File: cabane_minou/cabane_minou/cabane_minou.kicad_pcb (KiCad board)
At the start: 2 copper layers, 140 x 120.1 mm, 137 parts, among them J1 Alim 12V, J10 Serial, J11 LEDs Res, J12 Leds, J13 Buttons, J14 Couvercle, J15 Commande 12V, J2 Log, J3 Screen, J4 Bas, J5 LEDs Bas, J6 Move Tour, J7 LEDs Tour, J8 Move Haut, J9 LEDs Haut, Q1 BPC_2N2222A, Q10 BC327, Q11 BPC_2N2222A, Q12 BPC_2N2222A, Q13 BC327, Q14 BC327, Q2 BC327, Q3 BPC_2N2222A, Q4 BC327, Q5 BPC_2N2222A, Q6 BPC_IPP034N03L, Q7 BPC_2N2222A, Q8 BPC_2N2222A, Q9 BC327, U1 BPC_Alim5V, U2 LM1117DT-3.3, U3 BPC_ATMEGA2560_PRO, U5 RtcArduino, U6 BPC_ESP8266-01_ESP-01, X1 Trou, X2 Trou, X3 Trou, X4 Trou

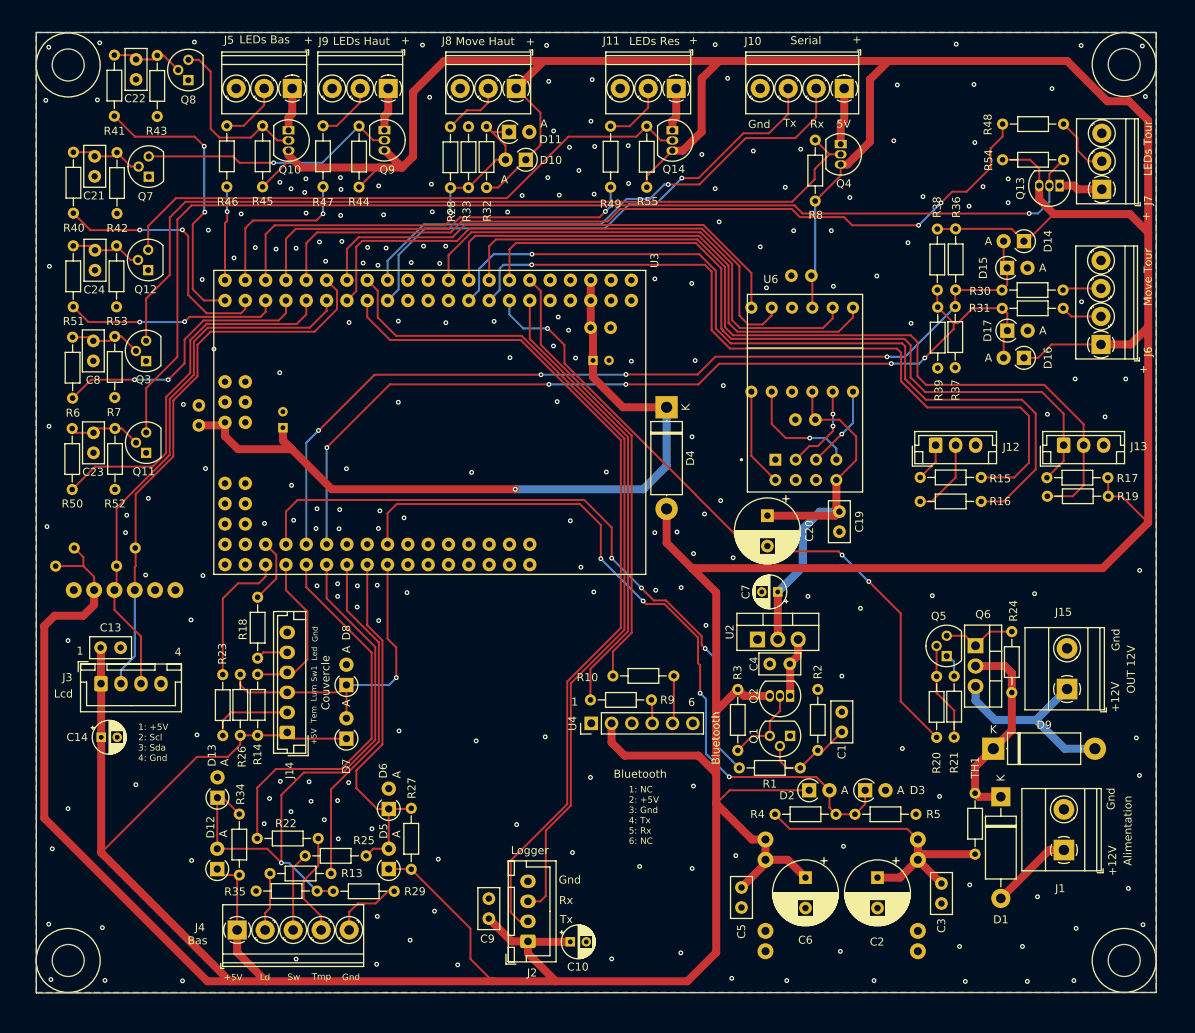
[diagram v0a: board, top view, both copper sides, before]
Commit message: Amélioration design du PCB (contour) Adaptation à la boîte Ajout datasheets
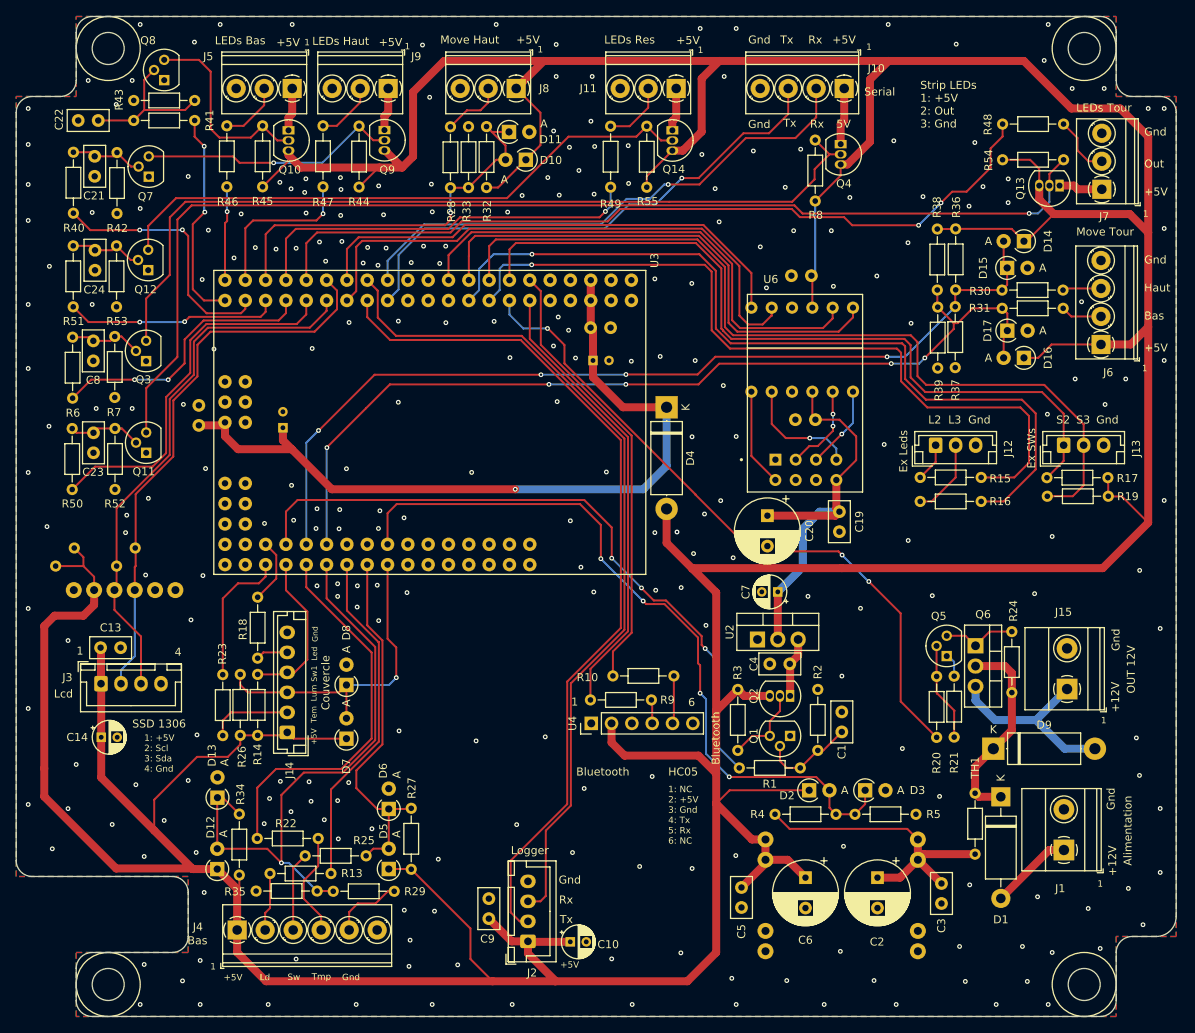
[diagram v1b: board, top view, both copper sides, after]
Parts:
- J4: footprint TerminalBlock_Phoenix:TerminalBlock_Phoenix_PT-1,5-5-3.5-H_1x05_P3.50mm_Horizontal -> TerminalBlock_Phoenix:TerminalBlock_Phoenix_PT-1,5-6-3.5-H_1x06_P3.50mm_Horizontal
- moved R41 10.1 mm to (93.8, 34.0), turned to 180 degrees
- moved C22 8.98 mm to (81.8, 34.0), turned to 180 degrees
- moved R43 7.32 mm to (93.8, 31.5), turned to 180 degrees
- moved X1 5.83 mm to (205.0, 142.0)
- moved X2 5.83 mm to (83.0, 142.0)
- moved X4 5.41 mm to (83.0, 25.0)
- moved X3 5.39 mm to (205.0, 25.0)
- moved Q8 3.02 mm to (90.0, 29.0)
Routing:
- net +5V: track 785.2 -> 749.6 mm
- net Net-(C22-Pad1): track 9.16 -> 18.6 mm
- net UC_5V_LEDS_BAS: track 35.9 -> 26.9 mm
- net Net-(Q10-B): track 22.1 -> 25.1 mm
- net GND: vias 216 -> 266
- net (no net): vias 1 -> 0
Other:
- board size 140 x 120.1 mm -> 145 x 125 mm
- board text added: "Ex Leds"
- board text added: "Ex SWs"
- board text added: "HC05"
- board text added: "Haut"
- board text added: "L2"
- board text added: "L3"
- board text added: "Out"
- board text added: "S2"
- board text added: "S3"
- board text added: "SSD 1306"
- board text added: "Strip LEDs 1: +5V 2: Out 3: Gnd"
- board text removed: "+"
